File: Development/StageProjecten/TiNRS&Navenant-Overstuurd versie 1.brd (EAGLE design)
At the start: 180.7 x 105.1 mm, 379 parts, among them IC1 7809DT, IC10 LM13700M, IC11 TL074TSSOP14, IC2 TL074TSSOP14, IC3 TL074TSSOP14, IC4 TL074TSSOP14, IC5 LM13700M, IC6 TL074TSSOP14, IC7 TL074TSSOP14, IC8 TL074TSSOP14, IC9 TL074TSSOP14, J1 JACK, J10 JACK, J11 JACK, J12 JACK, J13 JACK, J14 JACK, J15 JACK, J16 JACK, J17 JACK, J18 JACK, J19 JACK, J2 POWERSHROUDED, J20 JACK, J21 JACK, J22 JACK, J23 JACK, J24 JACK, J25 JACK, J26 JACK, J27 JACK, J3 JACK, J4 JACK, J5 JACK, J6 JACK, J7 JACK, J8 JACK, J9 JACK, Q1 MMBT3906LT1SMD, Q3 MMBT3906LT1SMD, Q4 MMBT3906LT1SMD, T1 3906, U1 LM358DR-1110010P1

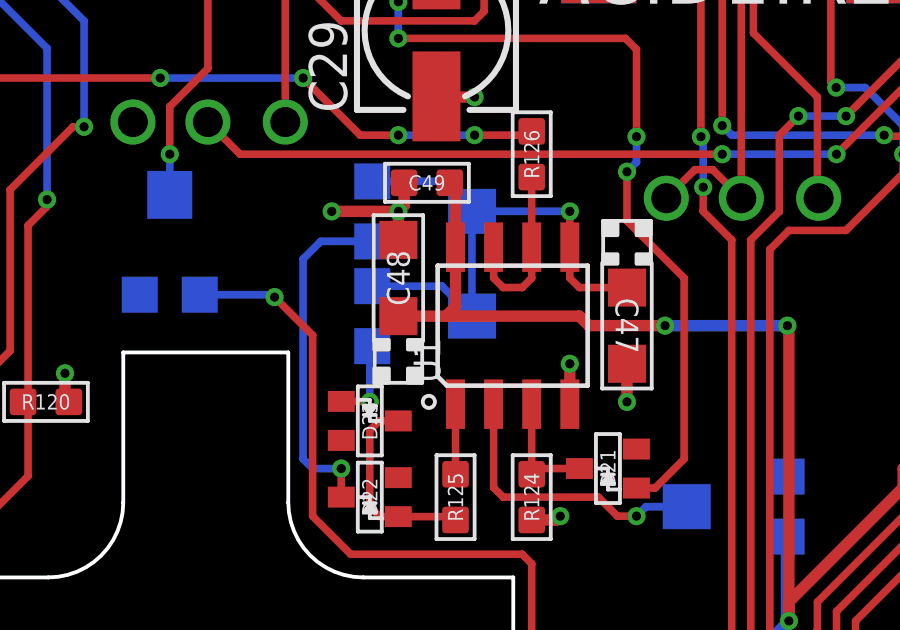
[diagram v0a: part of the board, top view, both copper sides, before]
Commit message: arboard los
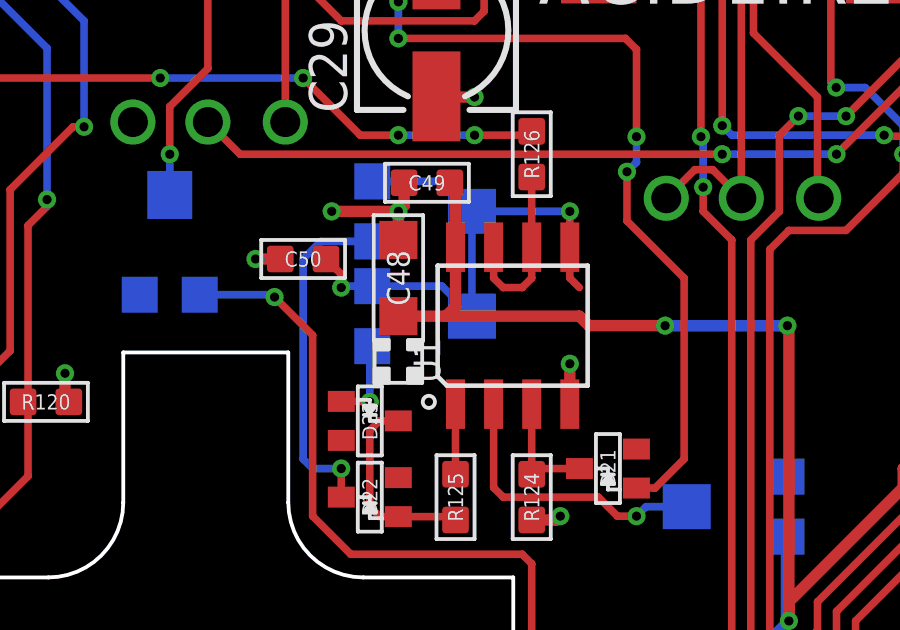
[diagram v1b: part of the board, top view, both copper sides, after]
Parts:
- removed C47: 10uF, EurorackModularParts:CASE-A_3216
- added C50: 22uF, OPL:C0603
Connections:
- net GND: now also C50.1; no longer C47.-
- net N$124: now also C50.2; no longer C47.+
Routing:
- net N$124: track 18.5 -> 19.1 mm, vias 1 -> 2
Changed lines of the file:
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@@
 <attribute name="VALUE" x="25.7175" y="32.385" size="1.27" layer="28" rot="MR180"/>
 </element>
-<element name="C47" library="EurorackModularParts" package="CASE-A_3216" value="10uF" x="34.29" y="28.8925" smashed="yes" rot="R270">
-<attribute name="NAME" x="34.29" y="28.8925" size="0.762" layer="25" ratio="10" rot="SR270" align="center"/>
-<attribute name="VALUE" x="32.798" y="30.4925" size="0.635" layer="27" ratio="10" rot="R270"/>
-</element>
 <element name="R126" library="OPL" package="R0603" value="1K" x="31.115" y="34.6075" smashed="yes" rot="R270">
 <attribute name="NAME" x="31.115" y="34.6075" size="0.508" layer="25" ratio="11" rot="R270" align="center"/>
@@
 <attribute name="VALUE" x="27.6225" y="32.7025" size="0.508" layer="27" ratio="10" align="top-center"/>
 </element>
+<element name="C50" library="OPL" package="C0603" value="22uF" x="23.495" y="31.115" smashed="yes">
+<attribute name="NAME" x="23.495" y="31.115" size="0.508" layer="25" ratio="11" align="center"/>
+<attribute name="VALUE" x="23.495" y="30.1625" size="0.508" layer="27" ratio="10" align="top-center"/>
+</element>
 </elements>
 <signals>
@@
 <contactref element="R124" pad="2"/>
 <contactref element="U$97" pad="1"/>
-<contactref element="C47" pad="-"/>
 <contactref element="C48" pad="-"/>
 <contactref element="C49" pad="1"/>
@@
 <wire x1="26.8605" y1="32.893" x2="26.67" y2="32.7025" width="0.381" layer="1"/>
 <wire x1="26.67" y1="31.75" x2="26.67" y2="32.7025" width="0.381" layer="1"/>
-<wire x1="34.29" y1="27.6225" x2="34.29" y2="26.3525" width="0.381" layer="1"/>
-<via x="34.29" y="26.3525" extent="1-16" drill="0.3048"/>
 <wire x1="32.385" y1="26.2763" x2="32.385" y2="27.6225" width="0.381" layer="1"/>
 <via x="32.385" y="27.6225" extent="1-16" drill="0.3048"/>
@@
 <wire x1="26.67" y1="32.7025" x2="24.4475" y2="32.7025" width="0.381" layer="1"/>
 <via x="24.4475" y="32.7025" extent="1-16" drill="0.3048"/>
+<contactref element="C50" pad="1"/>
+<wire x1="22.733" y1="31.115" x2="21.9075" y2="31.115" width="0.381" layer="1"/>
+<via x="21.9075" y="31.115" extent="1-16" drill="0.3048"/>
 </signal>
 <signal name="OUTPUT_A">
@@
 <contactref element="U$103" pad="2"/>
 <contactref element="U$103" pad="3"/>
-<contactref element="C47" pad="+"/>
 <contactref element="U1" pad="5"/>
 <wire x1="32.385" y1="31.5087" x2="32.385" y2="30.48" width="0.254" layer="1"/>
 <wire x1="32.385" y1="30.48" x2="32.7025" y2="30.1625" width="0.254" layer="1"/>
-<wire x1="32.7025" y1="30.1625" x2="34.29" y2="30.1625" width="0.254" layer="1"/>
 <wire x1="25.7975" y1="30.21" x2="28.1225" y2="30.21" width="0.254" layer="16"/>
 <wire x1="28.1225" y1="30.21" x2="29.1225" y2="29.21" width="0.254" layer="16"/>
@@
 <via x="32.385" y="32.7025" extent="1-16" drill="0.3048"/>
 <wire x1="32.385" y1="32.7025" x2="32.385" y2="31.5087" width="0.254" layer="1"/>
+<contactref element="C50" pad="2"/>
+<wire x1="24.257" y1="31.115" x2="24.765" y2="30.607" width="0.254" layer="1"/>
+<wire x1="24.765" y1="30.607" x2="24.765" y2="30.1625" width="0.254" layer="1"/>
+<via x="24.765" y="30.1625" extent="1-16" drill="0.3048"/>
+<wire x1="24.765" y1="30.1625" x2="24.8125" y2="30.21" width="0.254" layer="16"/>
+<wire x1="24.8125" y1="30.21" x2="25.7975" y2="30.21" width="0.254" layer="16"/>
 </signal>
 <signal name="N$123">
